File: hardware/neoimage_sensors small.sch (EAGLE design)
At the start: 34 parts, among them J8 AUDIO_JACK_3.5MM, U1 LIS3DH, U2 LIGHT_SENSORALS, U4 STM32F030F4P6TR, U6 LMV358

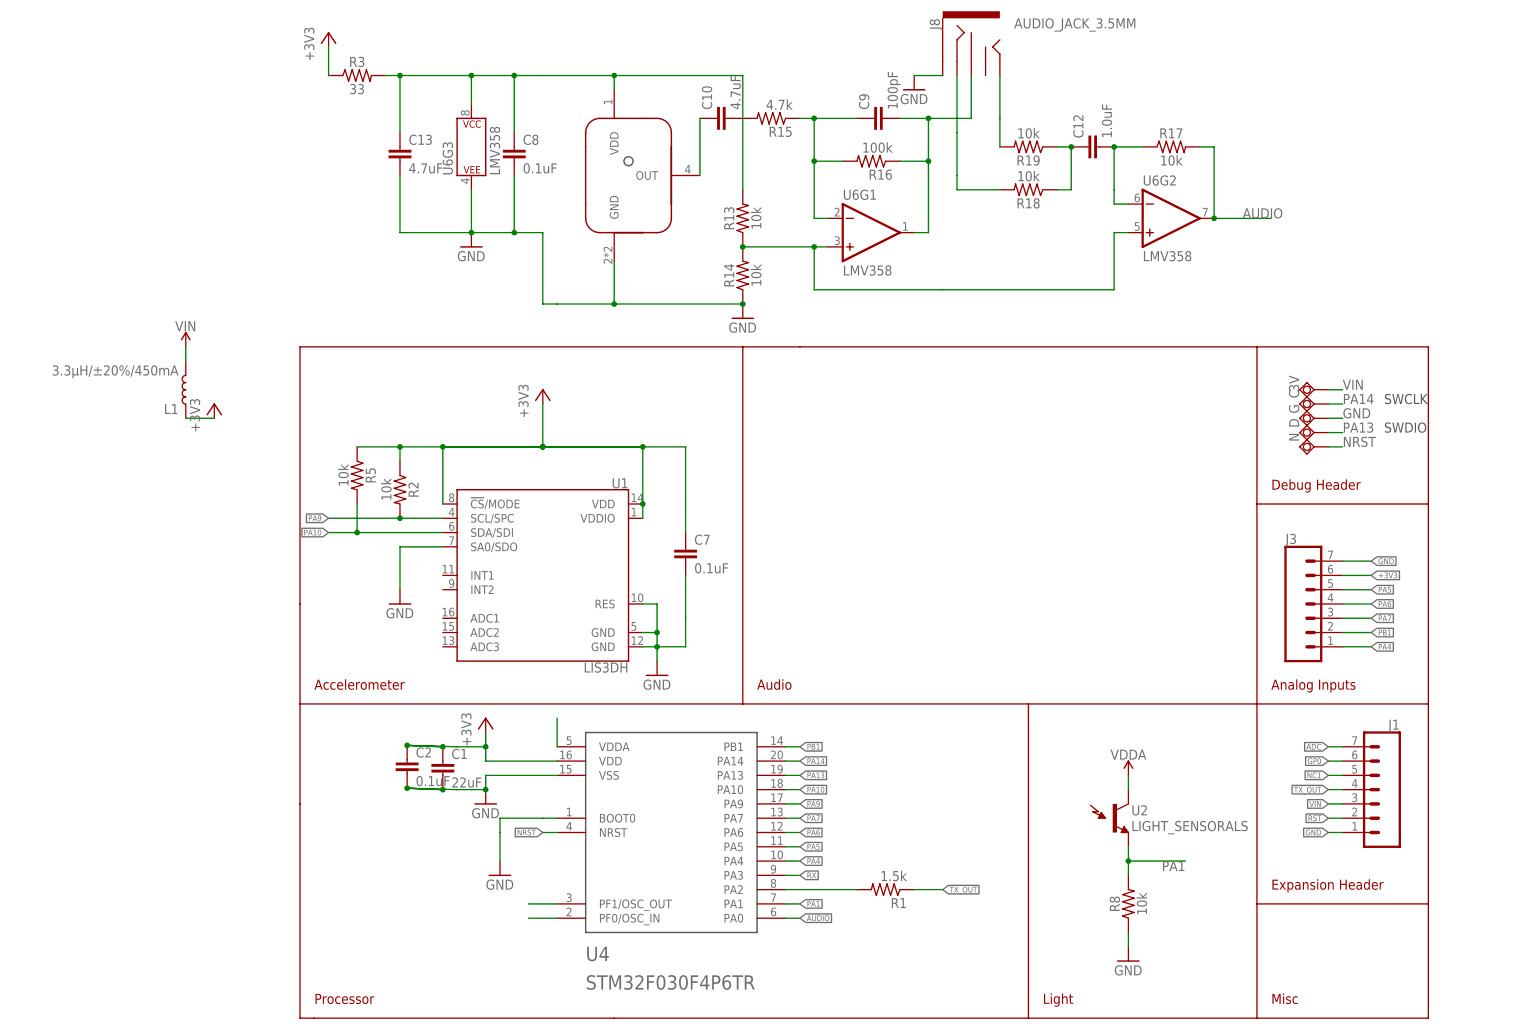
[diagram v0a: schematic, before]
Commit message: cleanup schematic, name signals, pdf
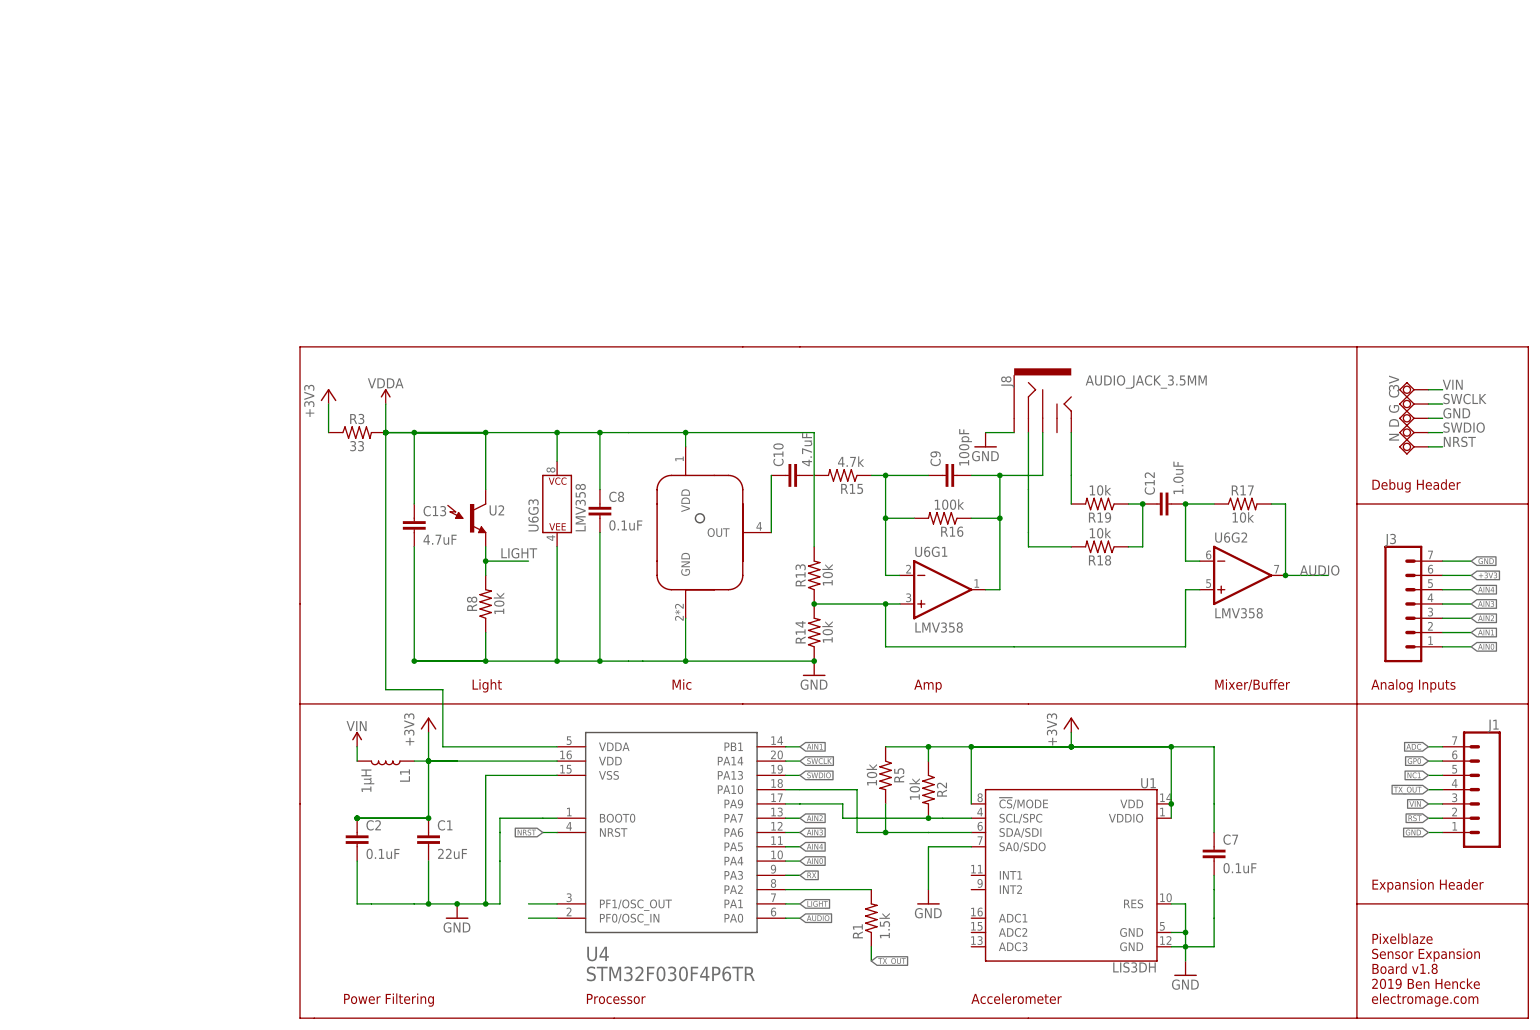
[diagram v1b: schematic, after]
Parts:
- L1: value 3.3µH/±20%/450mA -> 1µH
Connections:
- net PA1 renamed LIGHT
- net PA10 renamed SCL
- net PA13 renamed SWDIO
- net PA14 renamed SWCLK
- net PA4 renamed AIN0
- net PA5 renamed AIN4
- net PA6 renamed AIN3
- net PA7 renamed AIN2
- net PA9 renamed SDA
- net PB1 renamed AIN1
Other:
- note added: "Amp"
- note added: "Mic"
- note added: "Mixer/Buffer"
- note added: "Pixelblaze Sensor Expansion Board v1.8 2019 Ben Hencke electromage.com"
- note added: "Power Filtering"
- note removed: "Audio"
- note removed: "Misc"
- note removed: "SWCLK"
- note removed: "SWDIO"
- moved on the sheet: 3V, C, C1, C10, C12, C13, C2, C7, C8, C9, D, G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
